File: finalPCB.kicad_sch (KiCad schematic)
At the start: 71 parts, among them J1 9V Battery, J2 FCR7350R, J3 FCR7350R, J4 FCR7350R, J5 Switch, K1 HFD4/005, K2 HFD4/005, K3 HFD4/005, Q1 IRLML6401, Q2 IRLML6401, Q3 IRLML6401, Q4 IRLML6401, Q5 IRLML6401, Q6 NMOS, Q7 NMOS, Q8 NMOS, SW1 SW_Omron_B3FS, SW2 SW_Omron_B3FS, U1 7414, U1 ACS723xLCTR-05AB, U1 LMV358, U2 LMV358, U5 L7805

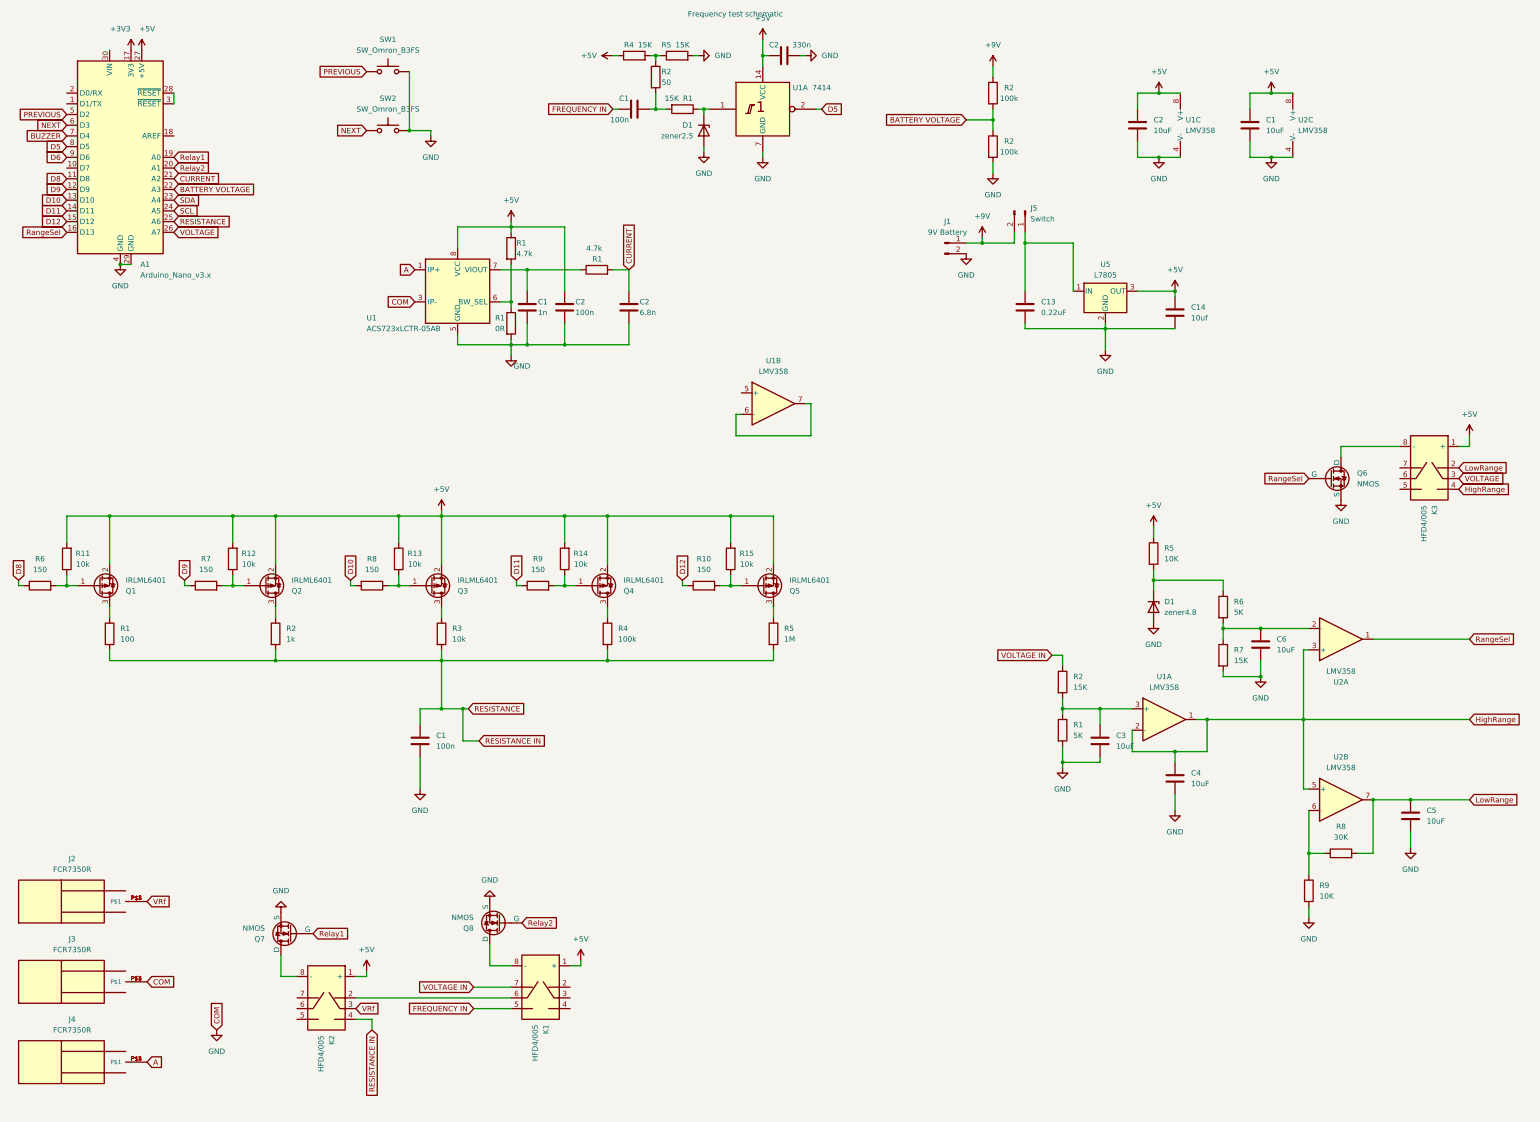
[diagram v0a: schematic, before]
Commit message: V1.0 Complete
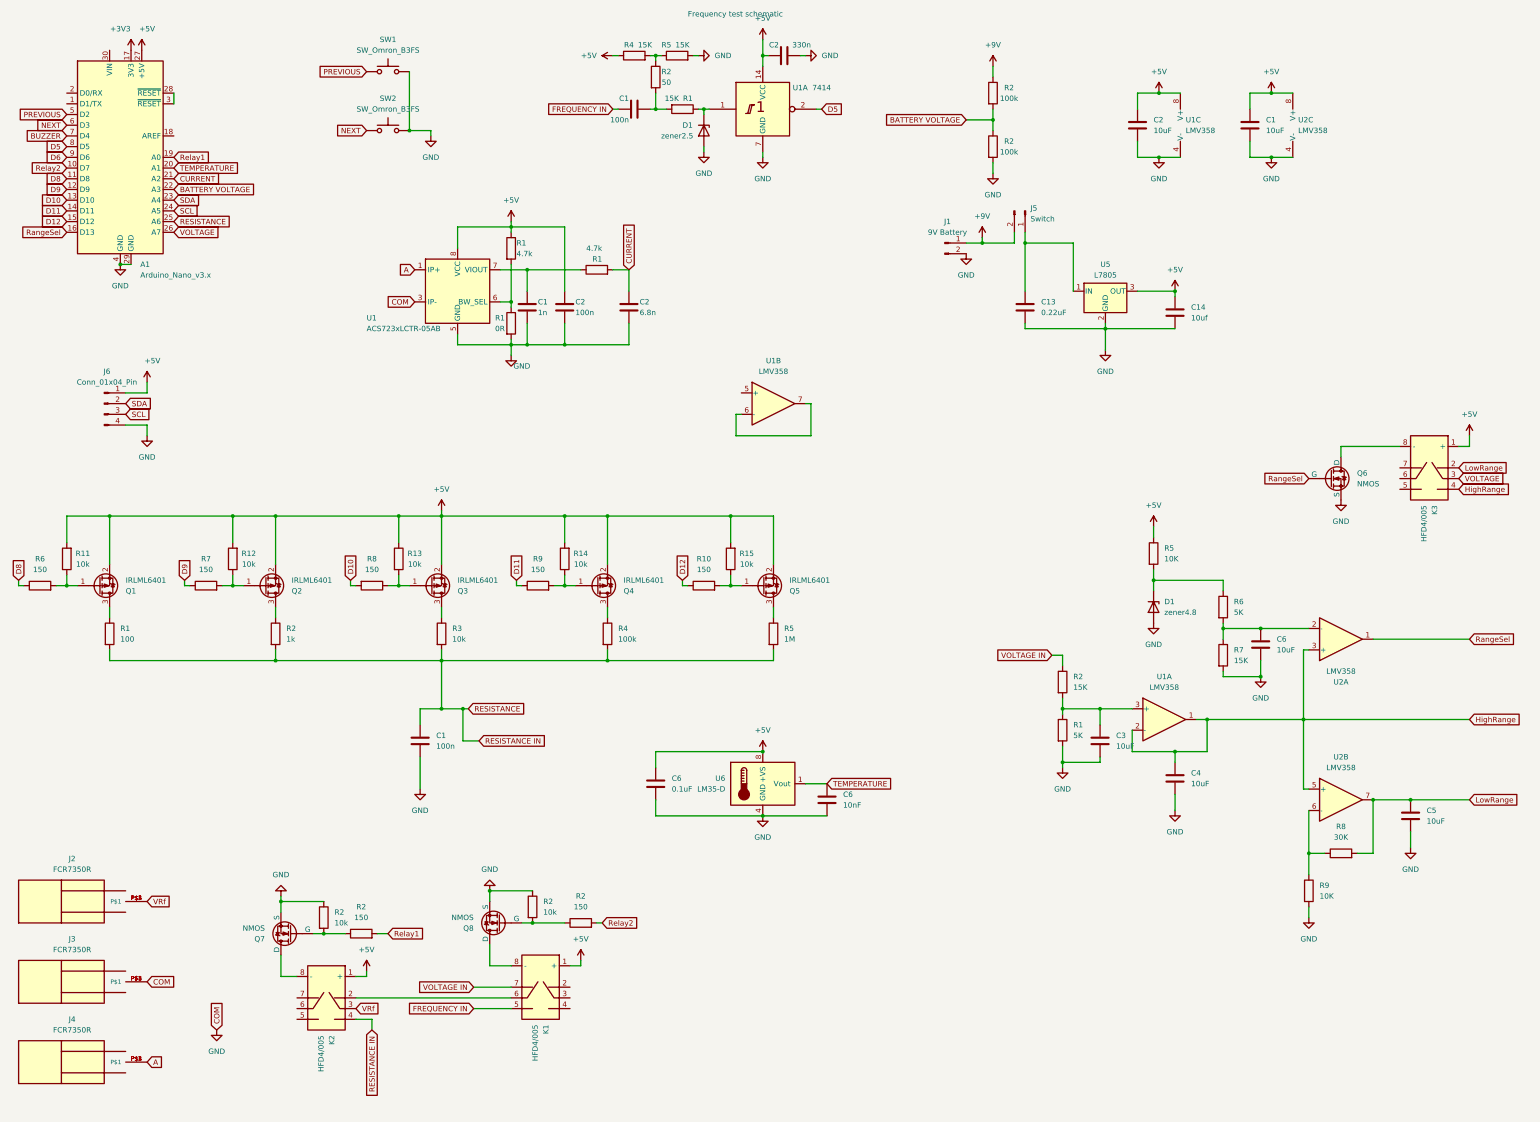
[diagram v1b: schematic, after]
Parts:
- added C6: 10nF, Capacitor_SMD:C_0805_2012Metric_Pad1.18x1.45mm_HandSolder, symbol Device:C
- added C6: 0.1uF, Capacitor_SMD:C_0805_2012Metric_Pad1.18x1.45mm_HandSolder, symbol Device:C
- added J6: Conn_01x04_Pin, Connector_JST:JST_XH_B4B-XH-AM_1x04_P2.50mm_Vertical, symbol Connector:Conn_01x04_Pin
- added R2 (x2): 10k, Resistor_SMD:R_0805_2012Metric_Pad1.20x1.40mm_HandSolder, symbol Device:R
- added R2 (x2): 150, Resistor_SMD:R_0805_2012Metric_Pad1.20x1.40mm_HandSolder, symbol Device:R
- added U6: LM35-D, Package_SO:SOIC-8_3.9x4.9mm_P1.27mm, symbol Sensor_Temperature:LM35-D
- J1, J5: footprint Connector_PinSocket_2.54mm:PinSocket_1x02_P2.54mm_Vertical -> Connector_JST:JST_XH_B2B-XH-AM_1x02_P2.50mm_Vertical
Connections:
- net +5V: now also C6.1, J6.1 (Pin_1), U6.8 (+VS)
- net GND: now also C6.2, C6.2, J6.4 (Pin_4), R2.1, R2.1, U6.4 (GND)
- net Relay1: now also R2.2; no longer Q7.2 (G)
- net Relay2: now also A1.10 (D7), R2.2; no longer A1.20 (A1), Q8.2 (G)
- net SCL: now also J6.3 (Pin_3)
- net SDA: now also J6.2 (Pin_2)
- new net: Q8.2 (G), R2.1, R2.2
- new net: Q7.2 (G), R2.1, R2.2
- new net TEMPERATURE: A1.20 (A1), C6.1, U6.1 (Vout)
